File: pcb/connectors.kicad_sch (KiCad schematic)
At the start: 5 parts, among them CN1 STDC14, CN2 SM04B-SRSS-TB (LF)(SN), CN4 SM04B-SRSS-TB (LF)(SN), J1 Conn_01x12, J2 Conn_01x16

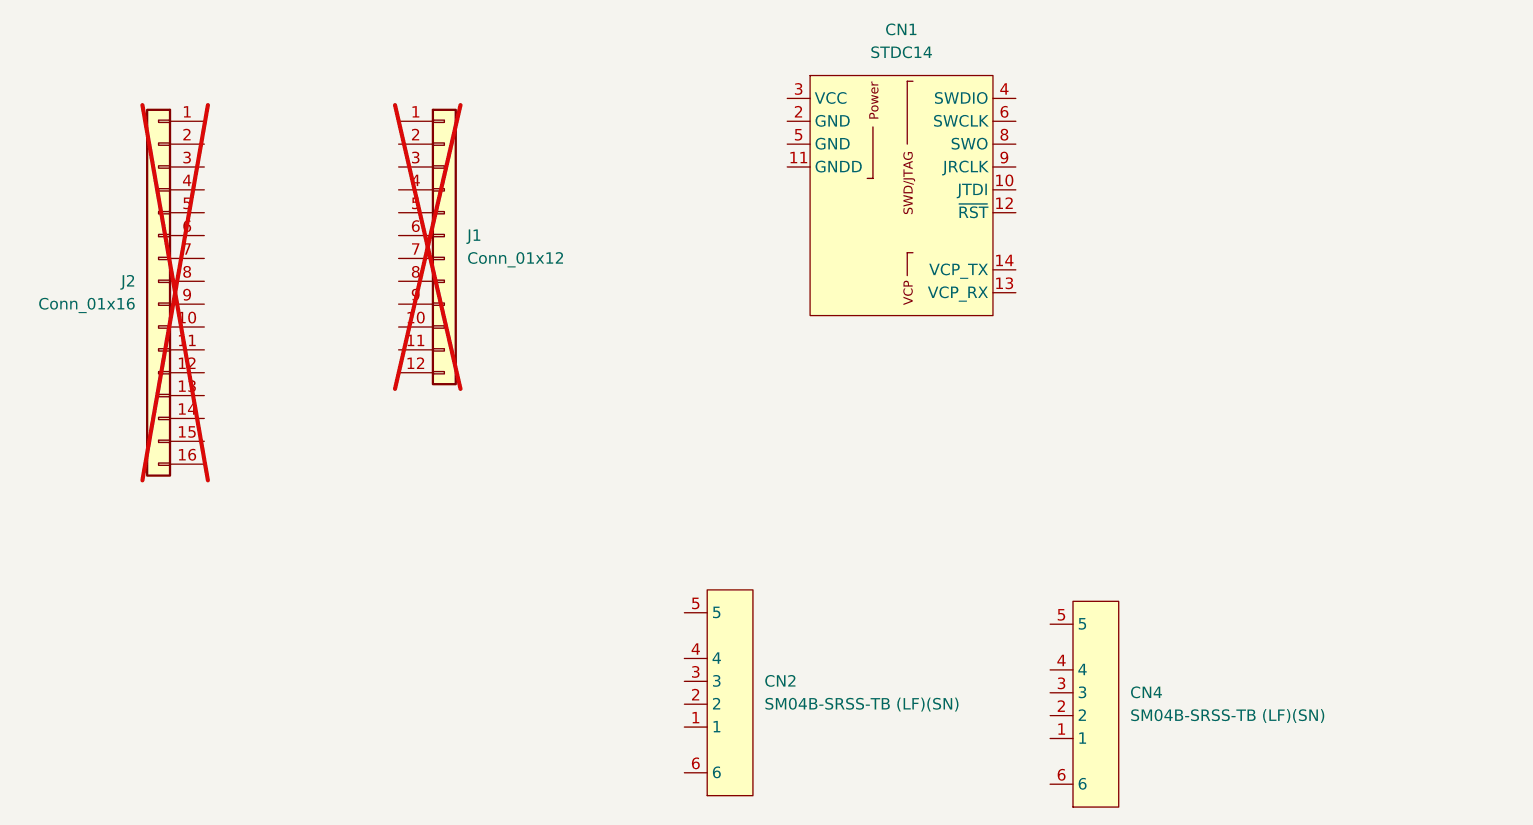
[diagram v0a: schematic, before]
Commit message: Work on schematics
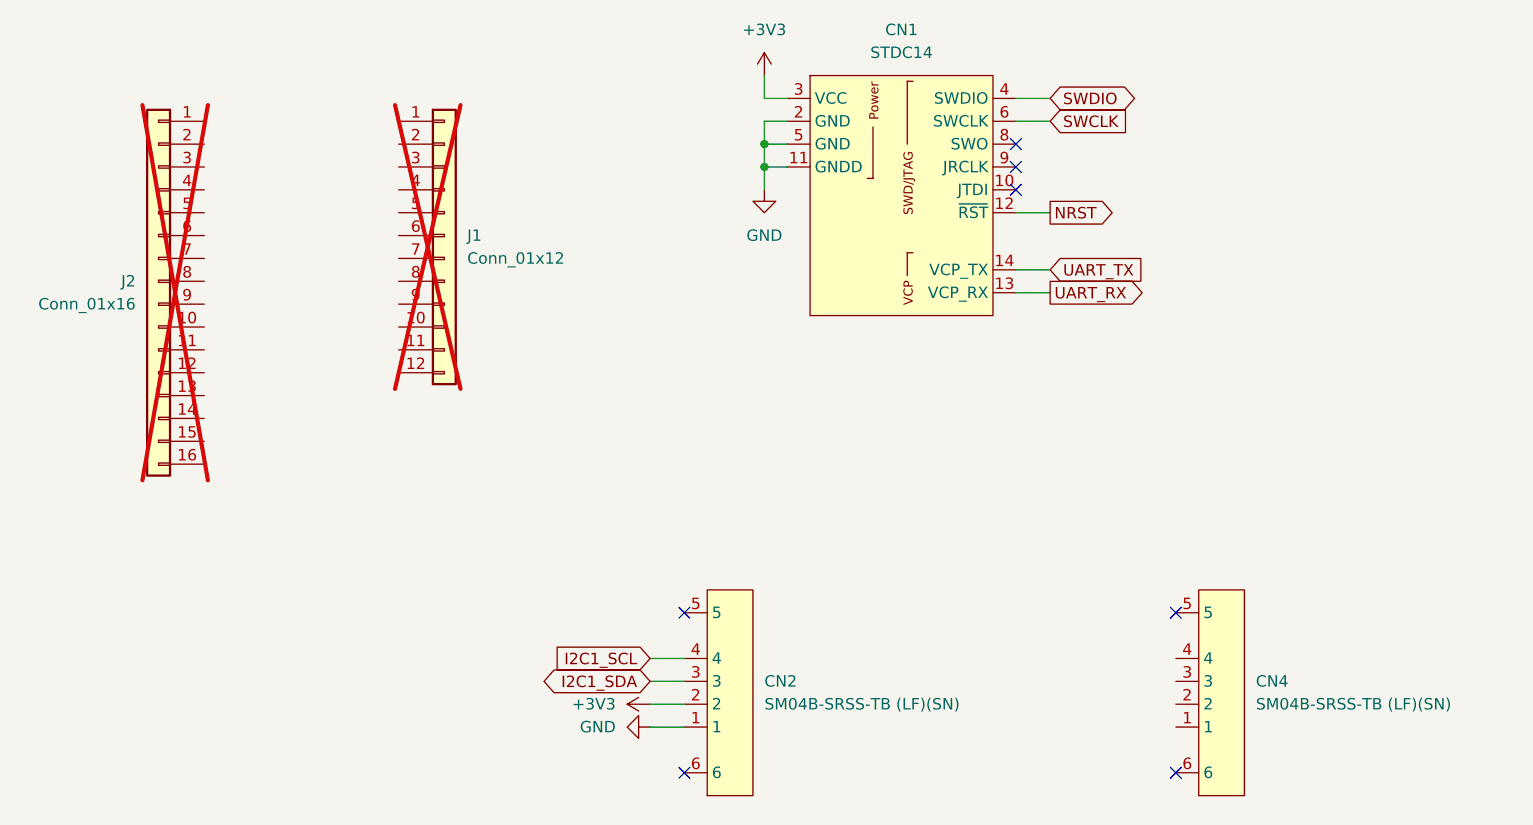
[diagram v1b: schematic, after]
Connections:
- net GND: now reaches CN2.1
- net GND: now also CN1.11 (GNDD), CN1.2 (GND), CN1.5 (GND)
- net +3V3: now reaches CN2.2
- net +3V3: now also CN1.3 (VCC)
- net I2C1_SDA: now reaches CN2.3
- net I2C1_SCL: now reaches CN2.4
- net NRST: now reaches CN1.12 (~{RST})
- net UART_RX: now reaches CN1.13 (VCP_RX)
- net UART_TX: now reaches CN1.14 (VCP_TX)
- net SWDIO: now reaches CN1.4 (SWDIO)
- net SWCLK: now reaches CN1.6 (SWCLK)
- no-connect marks 0 -> 7
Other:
- moved on the sheet: CN4
